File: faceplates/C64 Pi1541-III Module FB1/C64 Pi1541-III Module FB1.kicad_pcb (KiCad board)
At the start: 2 copper layers, 100 x 100 mm, 8 parts, among them M1 Mounting, M2 Mounting, M3 Mounting, M4 Mounting

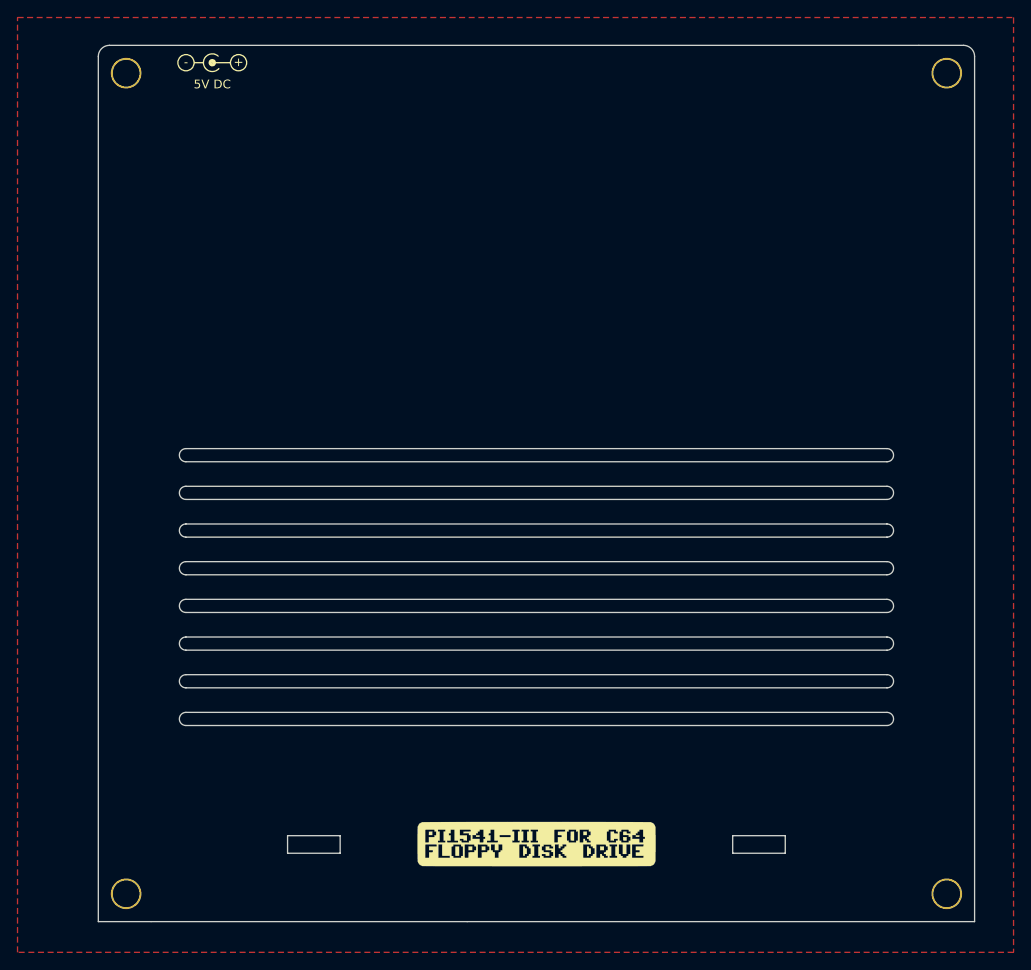
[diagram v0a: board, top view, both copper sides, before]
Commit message: ...
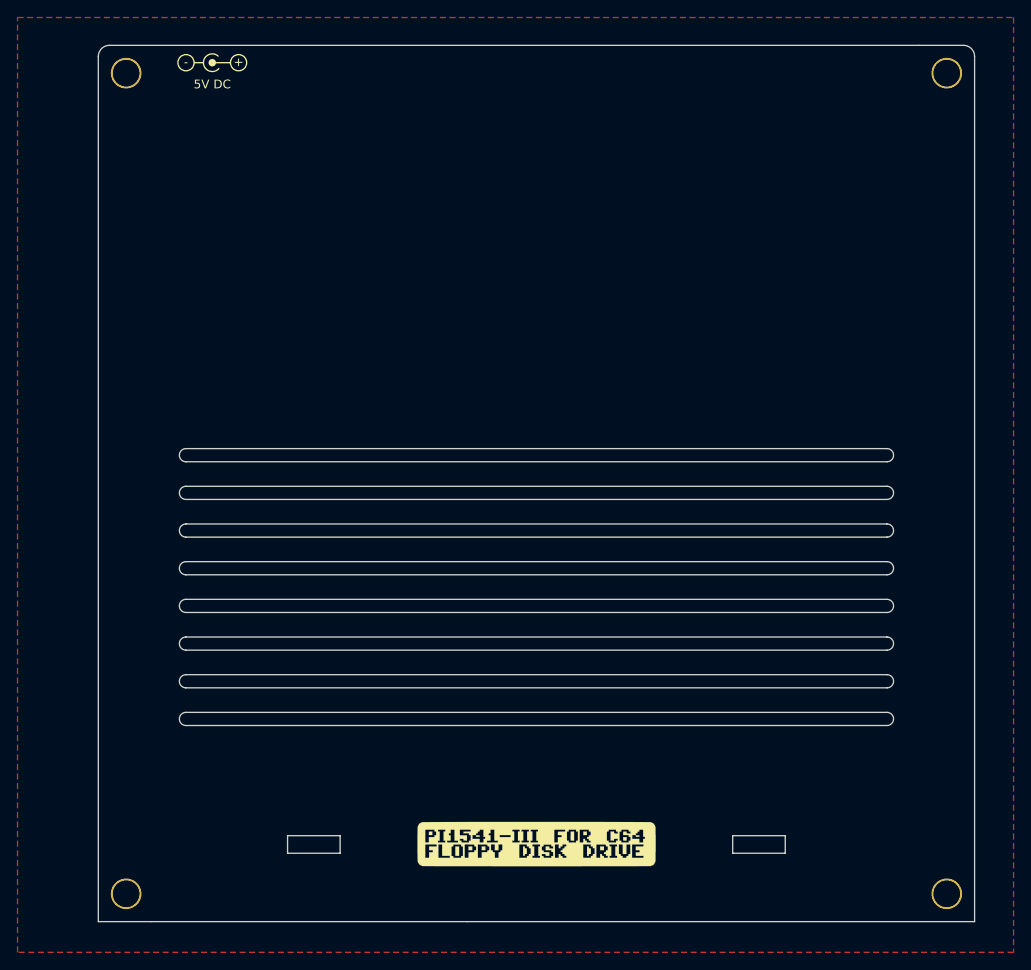
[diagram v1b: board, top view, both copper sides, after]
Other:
- net class Default removed
- net class Power removed
